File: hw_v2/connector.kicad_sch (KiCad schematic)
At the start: 22 parts, among them J1 Conn_02x24_Counter_Clockwise, J14 Conn_01x04, U11 L78M05ABDT-TR, U19 L78M05ABDT-TR, U25 74LVC2G17, U26 74LVC2G17, U8 AMS1117-3.3

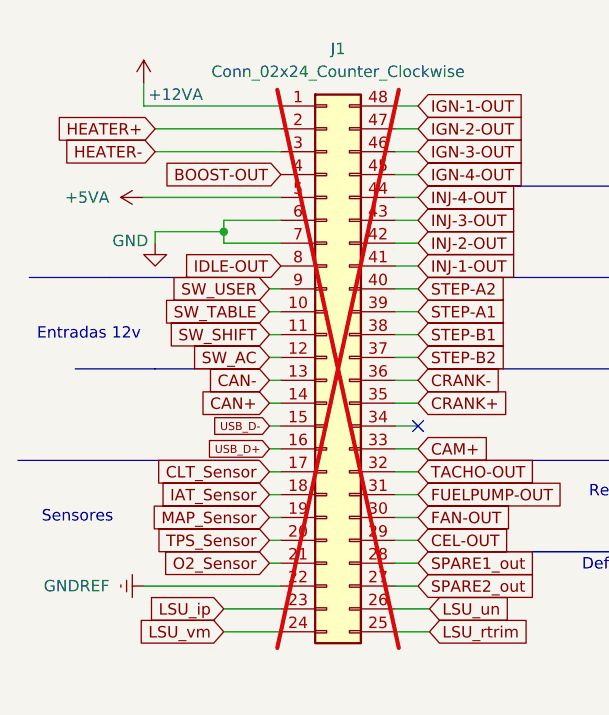
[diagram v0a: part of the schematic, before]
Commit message: wip analog frontend & power
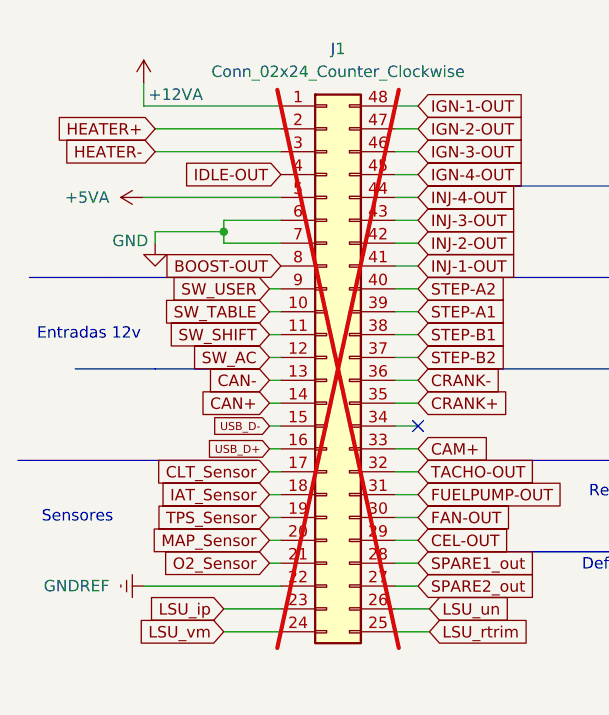
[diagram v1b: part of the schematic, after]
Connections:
- net BOOST-OUT: now also J1.8 (Pin_8); no longer J1.4 (Pin_4)
- net IDLE-OUT: now also J1.4 (Pin_4); no longer J1.8 (Pin_8)
- net MAP_Sensor: now also J1.20 (Pin_20); no longer J1.19 (Pin_19)
- net TPS_Sensor: now also J1.19 (Pin_19); no longer J1.20 (Pin_20)

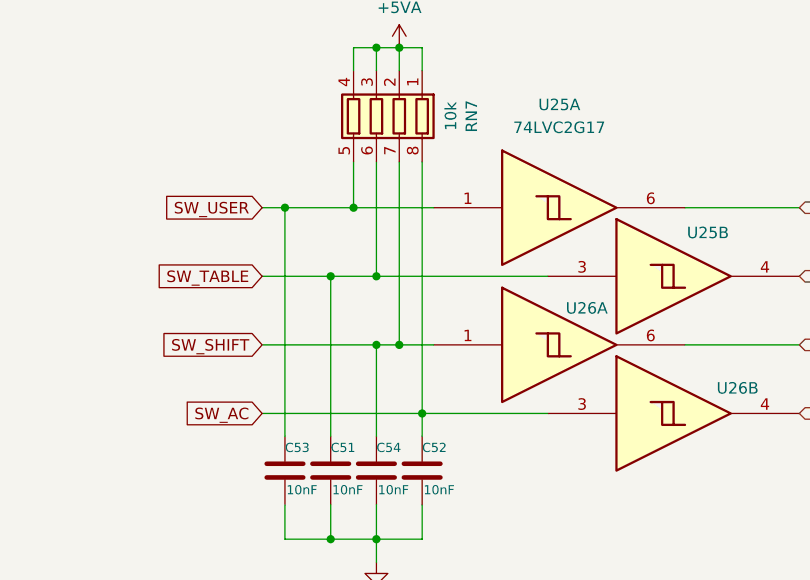
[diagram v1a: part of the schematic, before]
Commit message: wip analog frontend & power
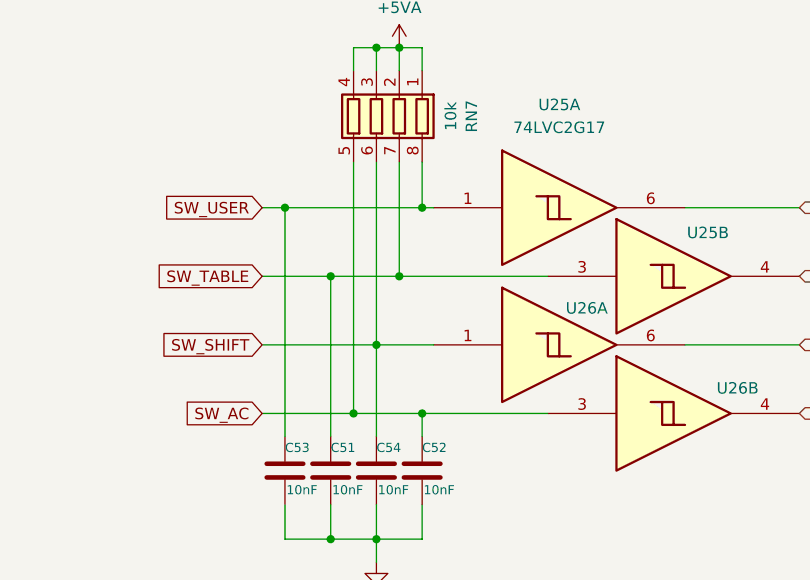
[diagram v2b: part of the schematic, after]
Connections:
- net SW_AC: now also RN7.5 (R4.2); no longer RN7.8 (R1.2)
- net SW_SHIFT: now also RN7.6 (R3.2); no longer RN7.7 (R2.2)
- net SW_TABLE: now also RN7.7 (R2.2); no longer RN7.6 (R3.2)
- net SW_USER: now also RN7.8 (R1.2); no longer RN7.5 (R4.2)
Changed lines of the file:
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@@
+	)
+	(junction
+		(at 214.63 97.79)
+		(diameter 0)
+		(color 0 0 0 0)
 	)
 	(junction
@@
 	)
 	(junction
+		(at 219.71 82.55)
+		(diameter 0)
+		(color 0 0 0 0)
+	)
+	(junction
 		(at 209.55 27.94)
 		(diameter 0)
@@
 	)
 	(junction
+		(at 222.25 74.93)
+		(diameter 0)
+		(color 0 0 0 0)
+	)
+	(junction
 		(at 217.17 90.17)
 		(diameter 0)
@@
 	)
 	(junction
-		(at 219.71 90.17)
-		(diameter 0)
-		(color 0 0 0 0)
-	)
-	(junction
-		(at 217.17 82.55)
-		(diameter 0)
-		(color 0 0 0 0)
-	)
-	(junction
 		(at 212.09 82.55)
-		(diameter 0)
-		(color 0 0 0 0)
-	)
-	(junction
-		(at 214.63 74.93)
 		(diameter 0)
 		(color 0 0 0 0)
@@
 	(wire
 		(pts
+			(xy 219.71 69.85) (xy 219.71 82.55)
+		)
+		(stroke
+			(width 0)
+			(type default)
+		)
+	)
+	(wire
+		(pts
 			(xy 217.17 114.3) (xy 217.17 111.76)
 		)
@@
 	(wire
 		(pts
+			(xy 212.09 82.55) (xy 219.71 82.55)
+		)
+		(stroke
+			(width 0)
+			(type default)
+		)
+	)
+	(wire
+		(pts
+			(xy 217.17 69.85) (xy 217.17 90.17)
+		)
+		(stroke
+			(width 0)
+			(type default)
+		)
+	)
+	(wire
+		(pts
 			(xy 195.58 31.75) (xy 195.58 30.48)
 		)
@@
 	(wire
 		(pts
-			(xy 219.71 90.17) (xy 223.52 90.17)
+			(xy 217.17 90.17) (xy 223.52 90.17)
 		)
 		(stroke
@@
 	(wire
 		(pts
+			(xy 214.63 69.85) (xy 214.63 97.79)
+		)
+		(stroke
+			(width 0)
+			(type default)
+		)
+	)
+	(wire
+		(pts
 			(xy 72.39 73.66) (xy 73.66 73.66)
 		)
@@
 	(wire
 		(pts
-			(xy 212.09 82.55) (xy 217.17 82.55)
-		)
-		(stroke
-			(width 0)
-			(type default)
-		)
-	)
-	(wire
-		(pts
 			(xy 222.25 35.56) (xy 222.25 39.37)
 		)
@@
 	(wire
 		(pts
+			(xy 222.25 74.93) (xy 223.52 74.93)
+		)
+		(stroke
+			(width 0)
+			(type default)
+		)
+	)
+	(wire
+		(pts
 			(xy 143.51 24.765) (xy 143.51 27.305)
 		)
@@
 	(wire
 		(pts
-			(xy 217.17 82.55) (xy 236.22 82.55)
-		)
-		(stroke
-			(width 0)
-			(type default)
-		)
-	)
-	(wire
-		(pts
 			(xy 217.17 57.15) (xy 219.71 57.15)
 		)
@@
 	(wire
 		(pts
-			(xy 219.71 69.85) (xy 219.71 90.17)
-		)
-		(stroke
-			(width 0)
-			(type default)
-		)
-	)
-	(wire
-		(pts
 			(xy 59.69 55.88) (xy 73.66 55.88)
 		)
@@
 		)
 	)
+	(wire
+		(pts
+			(xy 214.63 97.79) (xy 222.25 97.79)
+		)
+		(stroke
+			(width 0)
+			(type default)
+		)
+	)
 	(polyline
 		(pts
@@
 	(wire
 		(pts
-			(xy 214.63 69.85) (xy 214.63 74.93)
-		)
-		(stroke
-			(width 0)
-			(type default)
-		)
-	)
-	(wire
-		(pts
 			(xy 88.9 55.88) (xy 86.36 55.88)
 		)
@@
 		)
 	)
-	(wire
-		(pts
-			(xy 222.25 69.85) (xy 222.25 97.79)
-		)
-		(stroke
-			(width 0)
-			(type default)
-		)
-	)
 	(polyline
 		(pts
@@
 	(wire
 		(pts
+			(xy 222.25 69.85) (xy 222.25 74.93)
+		)
+		(stroke
+			(width 0)
+			(type default)
+		)
+	)
+	(wire
+		(pts
 			(xy 271.78 35.56) (xy 271.78 38.1)
 		)
@@
 	(wire
 		(pts
+			(xy 219.71 82.55) (xy 236.22 82.55)
+		)
+		(stroke
+			(width 0)
+			(type default)
+		)
+	)
+	(wire
+		(pts
 			(xy 143.51 40.005) (xy 143.51 38.1)
 		)
@@
 	(wire
 		(pts
-			(xy 207.01 74.93) (xy 214.63 74.93)
-		)
-		(stroke
-			(width 0)
-			(type default)
-		)
-	)
-	(wire
-		(pts
-			(xy 204.47 97.79) (xy 222.25 97.79)
-		)
-		(stroke
-			(width 0)
-			(type default)
-		)
-	)
-	(wire
-		(pts
-			(xy 214.63 74.93) (xy 223.52 74.93)
+			(xy 207.01 74.93) (xy 222.25 74.93)
+		)
+		(stroke
+			(width 0)
+			(type default)
+		)
+	)
+	(wire
+		(pts
+			(xy 204.47 97.79) (xy 214.63 97.79)
 		)
 		(stroke
@@
 	(wire
 		(pts
-			(xy 217.17 90.17) (xy 219.71 90.17)
-		)
-		(stroke
-			(width 0)
-			(type default)
-		)
-	)
-	(wire
-		(pts
 			(xy 222.25 111.76) (xy 222.25 107.95)
 		)
@@
 		)
 		(stroke
-			(width 0)
-			(type default)
-		)
-	)
-	(wire
-		(pts
-			(xy 217.17 69.85) (xy 217.17 82.55)
-		)
-		(stroke
